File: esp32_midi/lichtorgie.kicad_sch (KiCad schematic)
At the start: 64 parts

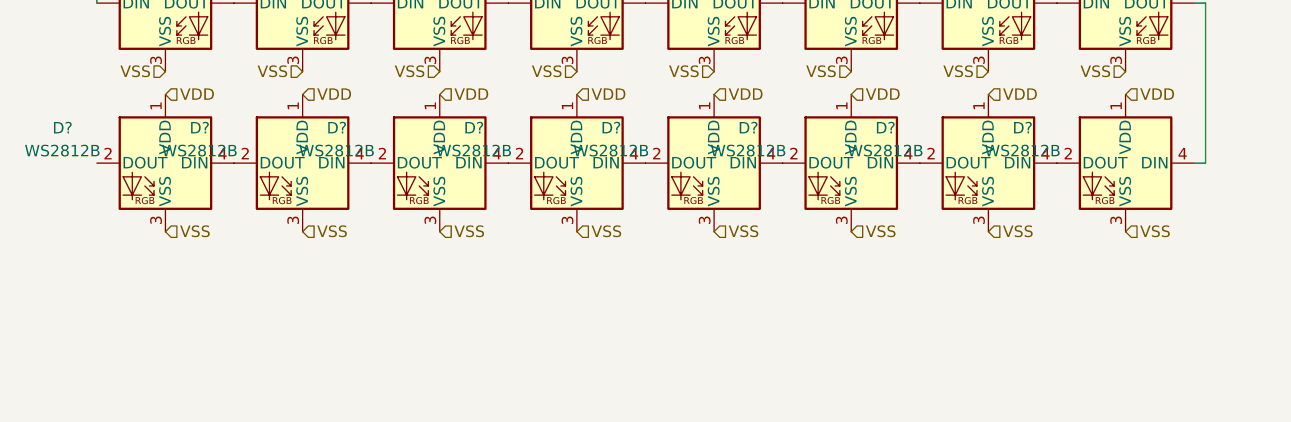
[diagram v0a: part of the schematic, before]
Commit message: Started work on PCB
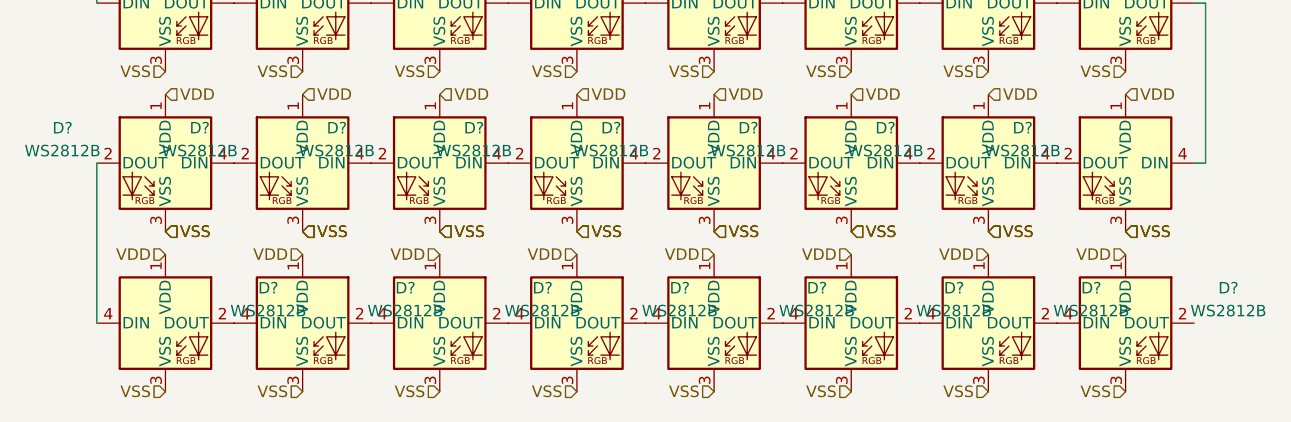
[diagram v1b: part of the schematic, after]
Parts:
- added D? (x8): WS2812B, LED_SMD:LED_WS2812B_PLCC4_5.0x5.0mm_P3.2mm, symbol LED:WS2812B
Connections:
- net VDD: now also D?.1 (VDD), D?.1 (VDD), D?.1 (VDD), D?.1 (VDD), D?.1 (VDD), D?.1 (VDD), D?.1 (VDD), D?.1 (VDD)
- net VSS: now also D?.3 (VSS), D?.3 (VSS), D?.3 (VSS), D?.3 (VSS), D?.3 (VSS), D?.3 (VSS), D?.3 (VSS), D?.3 (VSS)
- net at D?.2 (DOUT): now also D?.4 (DIN)
- new net: D?.2 (DOUT), D?.4 (DIN) (x7)
